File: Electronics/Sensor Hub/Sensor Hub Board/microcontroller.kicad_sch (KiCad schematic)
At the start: 57 parts, among them IC301 STM32H723ZGT6, IC302 TJA1057GT/3, IC303 TJA1057GT/3, IC304 TJA1057GT/3, J301 TC2030, J302 MEM2075-00-140-01-A, J303 TYPE-C-31-M-12, J304 Screw_Terminal_01x02, J305 Screw_Terminal_01x02, J306 Screw_Terminal_01x02, SW301 SW_DIP_x02, U301 USBLC6-4SC6-ES, U302 USBLC6-4SC6-ES, X301 25MHz_Clock, X302 25MHz_Clock, X303 32.768kHz_Clock

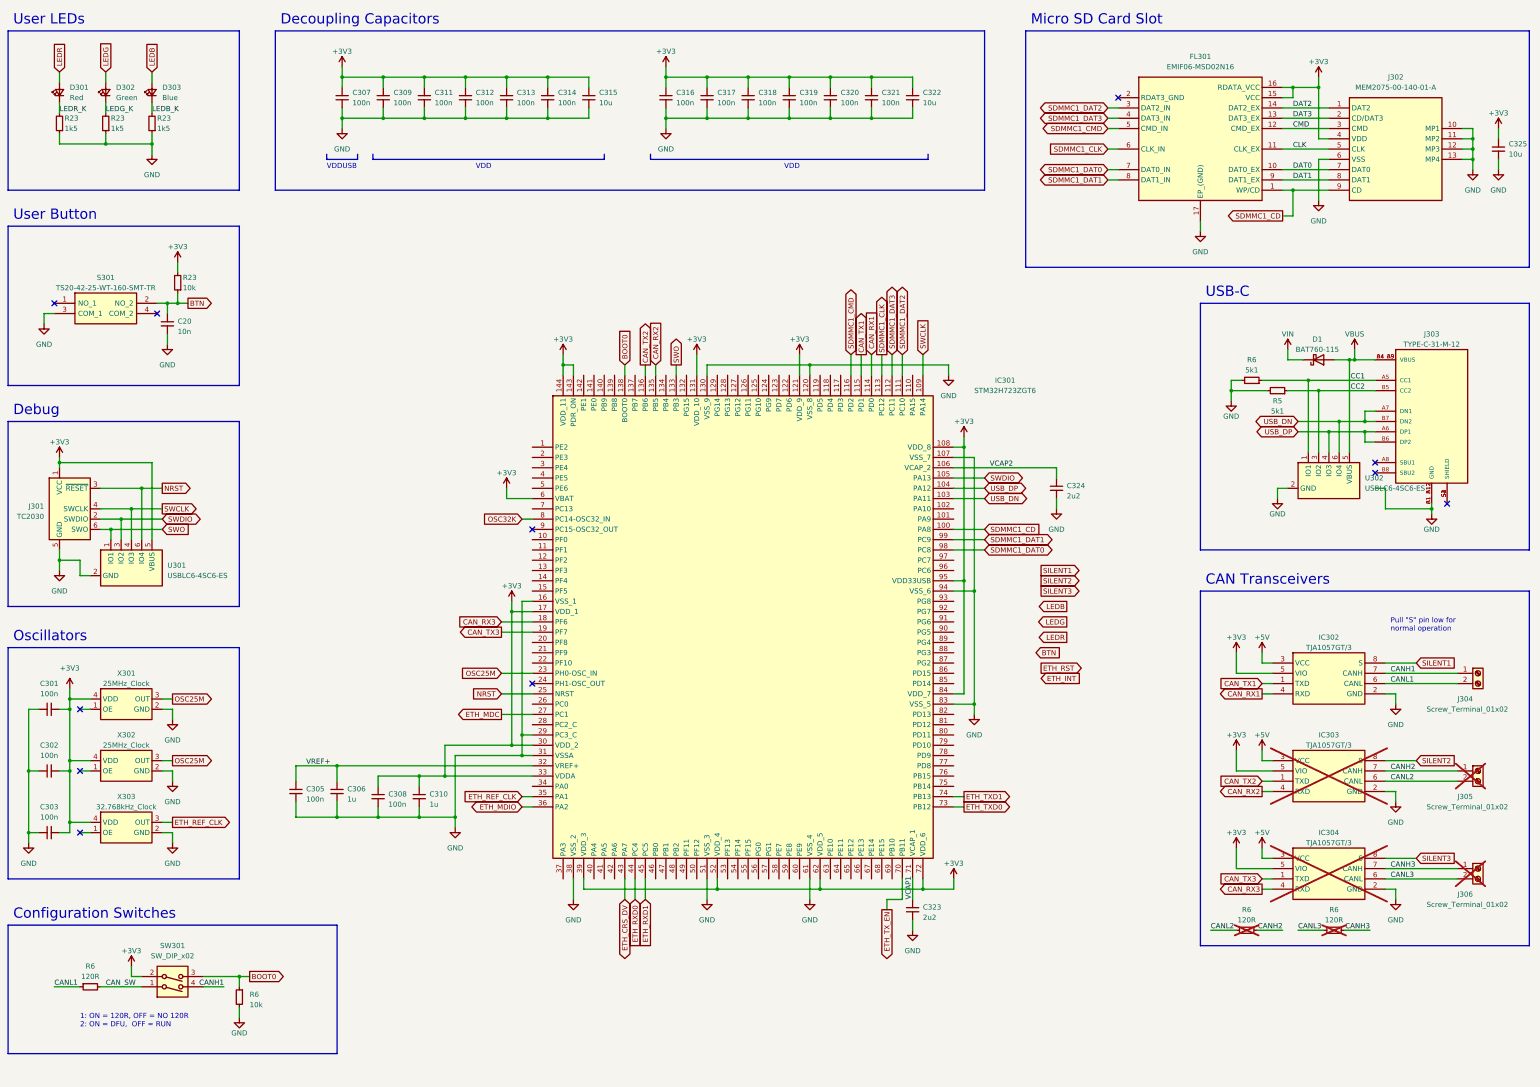
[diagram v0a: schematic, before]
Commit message: PCB Schematics finished
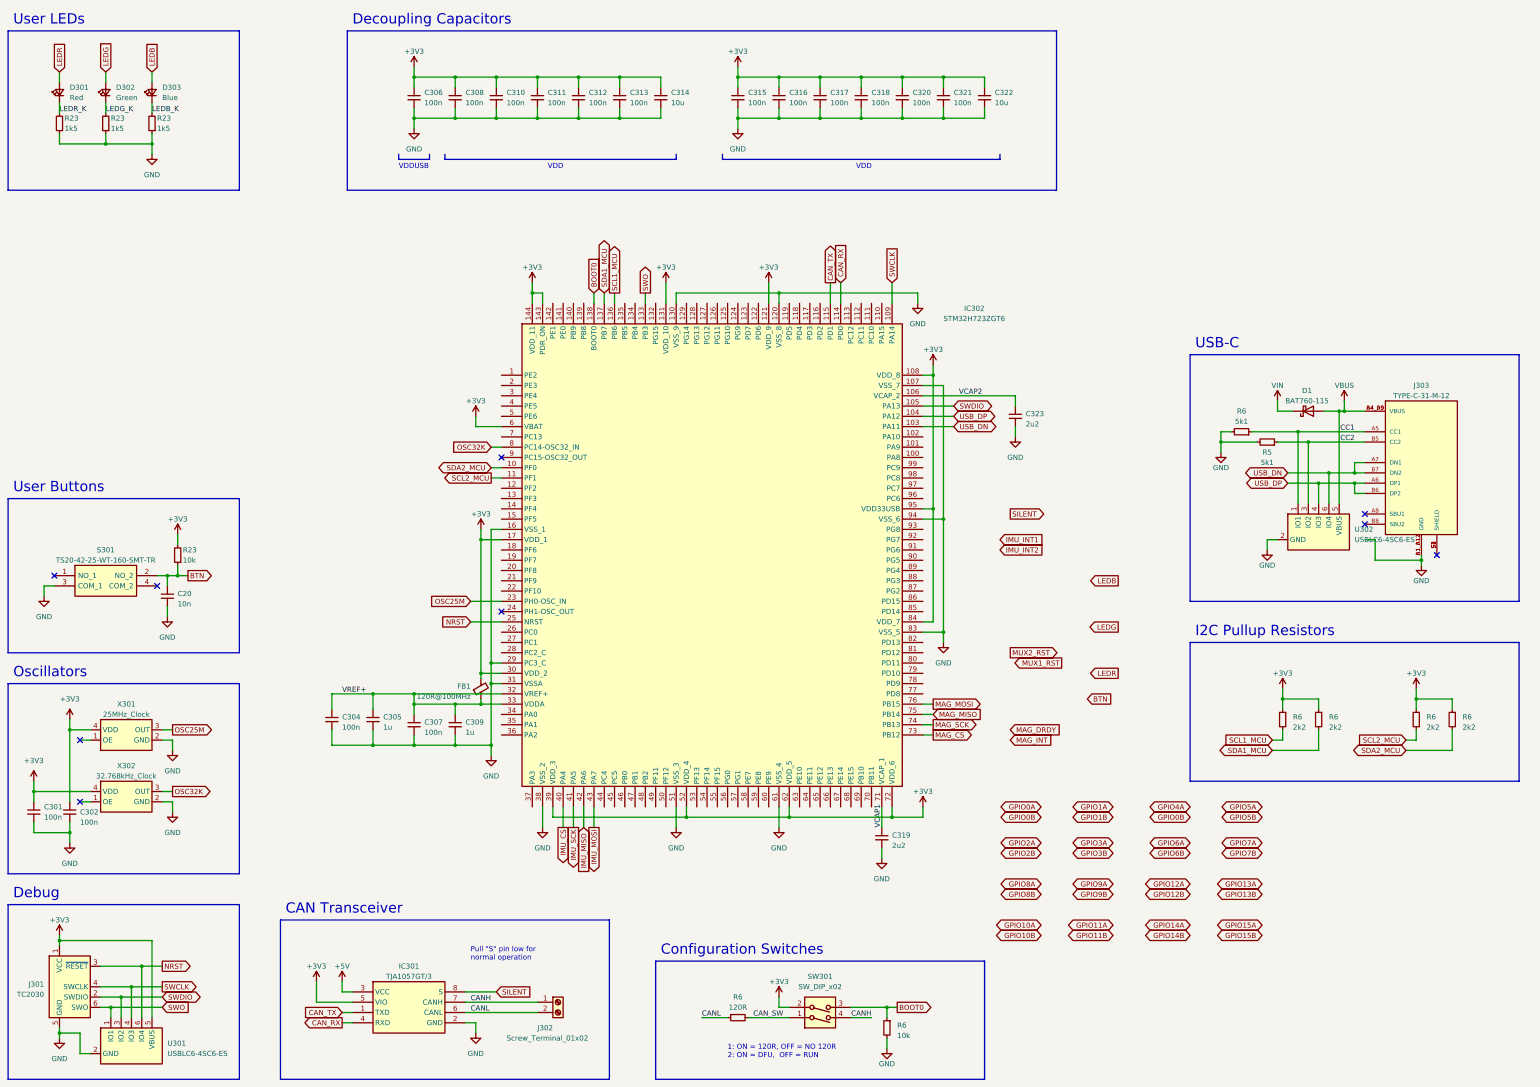
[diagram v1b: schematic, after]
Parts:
- removed C301: 100n, Capacitor_SMD:C_0402_1005Metric, symbol Device:C_Small
- removed C325: 10u, Capacitor_SMD:C_0402_1005Metric, symbol Device:C_Small
- removed FL301: EMIF06-MSD02N16, EMIF06MSD02N16, symbol EMIF06-MSD02N16:EMIF06-MSD02N16
- removed IC303, IC304: TJA1057GT/3, SOIC127P600X175-8N, symbol TJA1057T:TJA1057GT/3
- removed J302: MEM2075-00-140-01-A, MEM20750014001A, symbol MEM2075-00-140-01-A:MEM2075-00-140-01-A
- removed J305, J306: Screw_Terminal_01x02, TerminalBlock:TerminalBlock_bornier-2_P5.08mm, symbol Connector:Screw_Terminal_01x02
- removed R6: 5k1, Resistor_SMD:R_0402_1005Metric, symbol Device:R_Small
- removed R6 (x2): 120R, Resistor_SMD:R_0402_1005Metric, symbol Device:R_Small
- removed X301: 25MHz_Clock, Oscillator:Oscillator_SMD_Abracon_ASE-4Pin_3.2x2.5mm_HandSoldering, symbol MSL_Symbols:25MHz_Clock
- added FB1: 120R@100MHz, Resistor_SMD:R_0402_1005Metric, symbol Device:FerriteBead_Small
- added R6: 5k1, Resistor_SMD:R_0402_1005Metric, symbol Device:R_Small
- added R6 (x4): 2k2, Resistor_SMD:R_0402_1005Metric, symbol Device:R_Small
- renumbered C303 to C301, C305 to C304, C306 to C305, C307 to C306, C308 to C307, C309 to C308, C310 to C309, C311 to C310, C312 to C311, C313 to C312, C314 to C313, C315 to C314, C316 to C315, C317 to C316, C318 to C317, C319 to C318, C323 to C319, C324 to C323, IC302 to IC301, IC301 to IC302, J304 to J302, X302 to X301, X303 to X302
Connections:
- net +3V3: now also C301.1, FB1.2, R6.1, R6.1, R6.1, R6.1; no longer C301.2, C307.1, C309.1, IC302.33 (VDDA)
- net CC1: now also R6.1
- net GND: now also C301.2, R6.2; no longer C301.1
- net OSC32K: now also X302.3 (OUT)
- net VREF+: now also C307.1, C309.1, IC302.33 (VDDA), FB1.1
- net SDA2_MCU: now reaches IC302.10 (PF0)
- net SDA2_MCU: now also R6.2
- net SCL2_MCU: now reaches IC302.11 (PF1)
- net SCL2_MCU: now also R6.2
- net SDA1_MCU: now reaches IC302.137 (PB7)
- net SDA1_MCU: now also R6.2
- net IMU_CS: now reaches IC302.40 (PA4)
- net IMU_SCK: now reaches IC302.41 (PA5)
- net IMU_MISO: now reaches IC302.42 (PA6)
- net MAG_MISO: now reaches IC302.75 (PB14)
- net MAG_MOSI: now reaches IC302.76 (PB15)
- net CANH1 renamed CANH
- net CANL1 renamed CANL
- net CAN_RX1 renamed CAN_RX
- net CAN_RX2: no longer names the net of IC302.135 (PB5)
- net CAN_RX3: no longer names the net of IC302.18 (PF6)
- net CAN_TX1 renamed CAN_TX
- net CAN_TX2 renamed SCL1_MCU
- net SCL1_MCU: now also R6.2
- net CAN_TX3: no longer names the net of IC302.19 (PF7)
- net ETH_CRS_DV renamed IMU_MOSI
- net ETH_MDC: no longer names the net of IC302.27 (PC1)
- net ETH_MDIO: no longer names the net of IC302.36 (PA2)
- net ETH_REF_CLK: no longer names the net of IC302.35 (PA1)
- net ETH_REF_CLK: no longer X302.3 (OUT)
- net ETH_RXD0: no longer names the net of IC302.44 (PC4)
- net ETH_RXD1: no longer names the net of IC302.45 (PC5)
- net ETH_TXD0 renamed MAG_CS
- net ETH_TXD1 renamed MAG_SCK
- net ETH_TX_EN: no longer names the net of IC302.70 (PB11)
- net SDMMC1_CD: no longer names the net of IC302.100 (PA8)
- net SDMMC1_CLK: no longer names the net of IC302.113 (PC12)
- net SDMMC1_CMD: no longer names the net of IC302.116 (PD2)
- net SDMMC1_DAT0: no longer names the net of IC302.98 (PC8)
- net SDMMC1_DAT1: no longer names the net of IC302.99 (PC9)
- net SDMMC1_DAT2: no longer names the net of IC302.111 (PC10)
- net SDMMC1_DAT3: no longer names the net of IC302.112 (PC11)
- net SILENT1 renamed SILENT
- no-connect marks 11 -> 9
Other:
- note added: "CAN Transceiver"
- note added: "I2C Pullup Resistors"
- note added: "User Buttons"
- note removed: "CAN Transceivers"
- note removed: "Micro SD Card Slot"
- note removed: "User Button"
- moved on the sheet: C301, C304, C305, C306, C307, C308, C309, C310, C311, C312, C313, C314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
